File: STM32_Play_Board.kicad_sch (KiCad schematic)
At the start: 0 parts

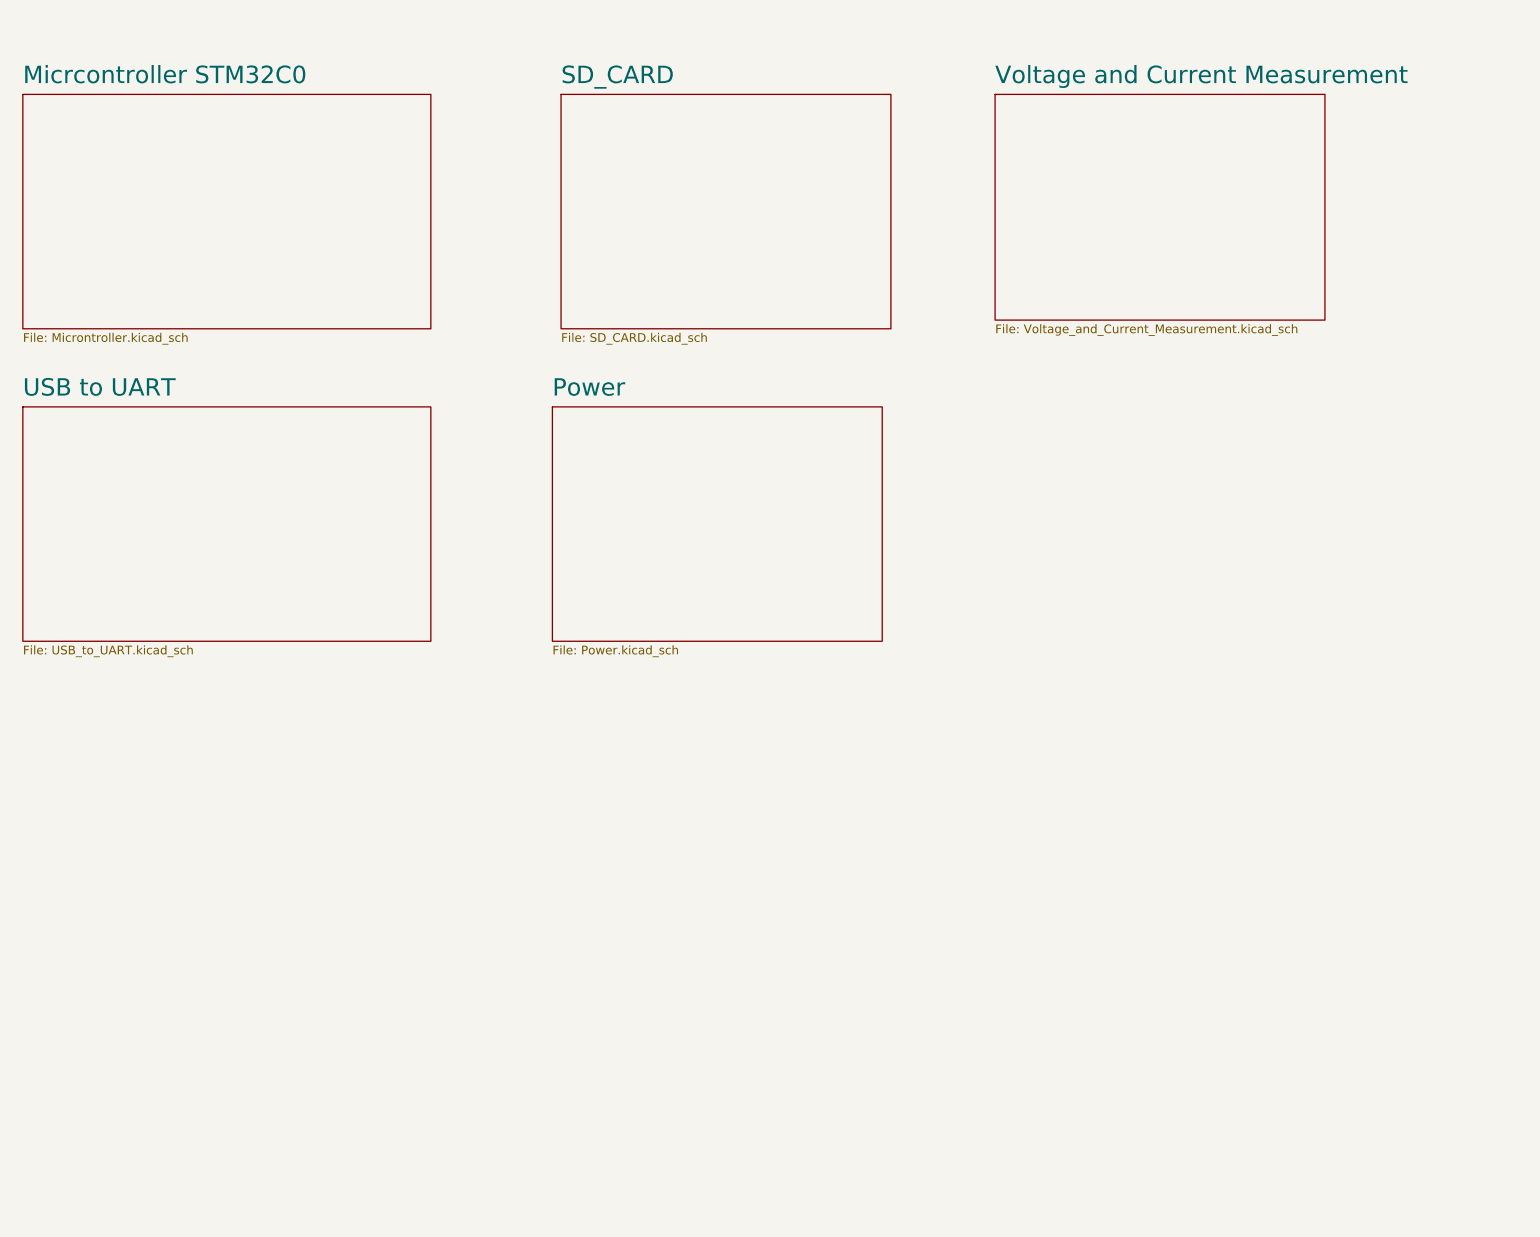
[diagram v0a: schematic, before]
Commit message: changes to schematic and PCB
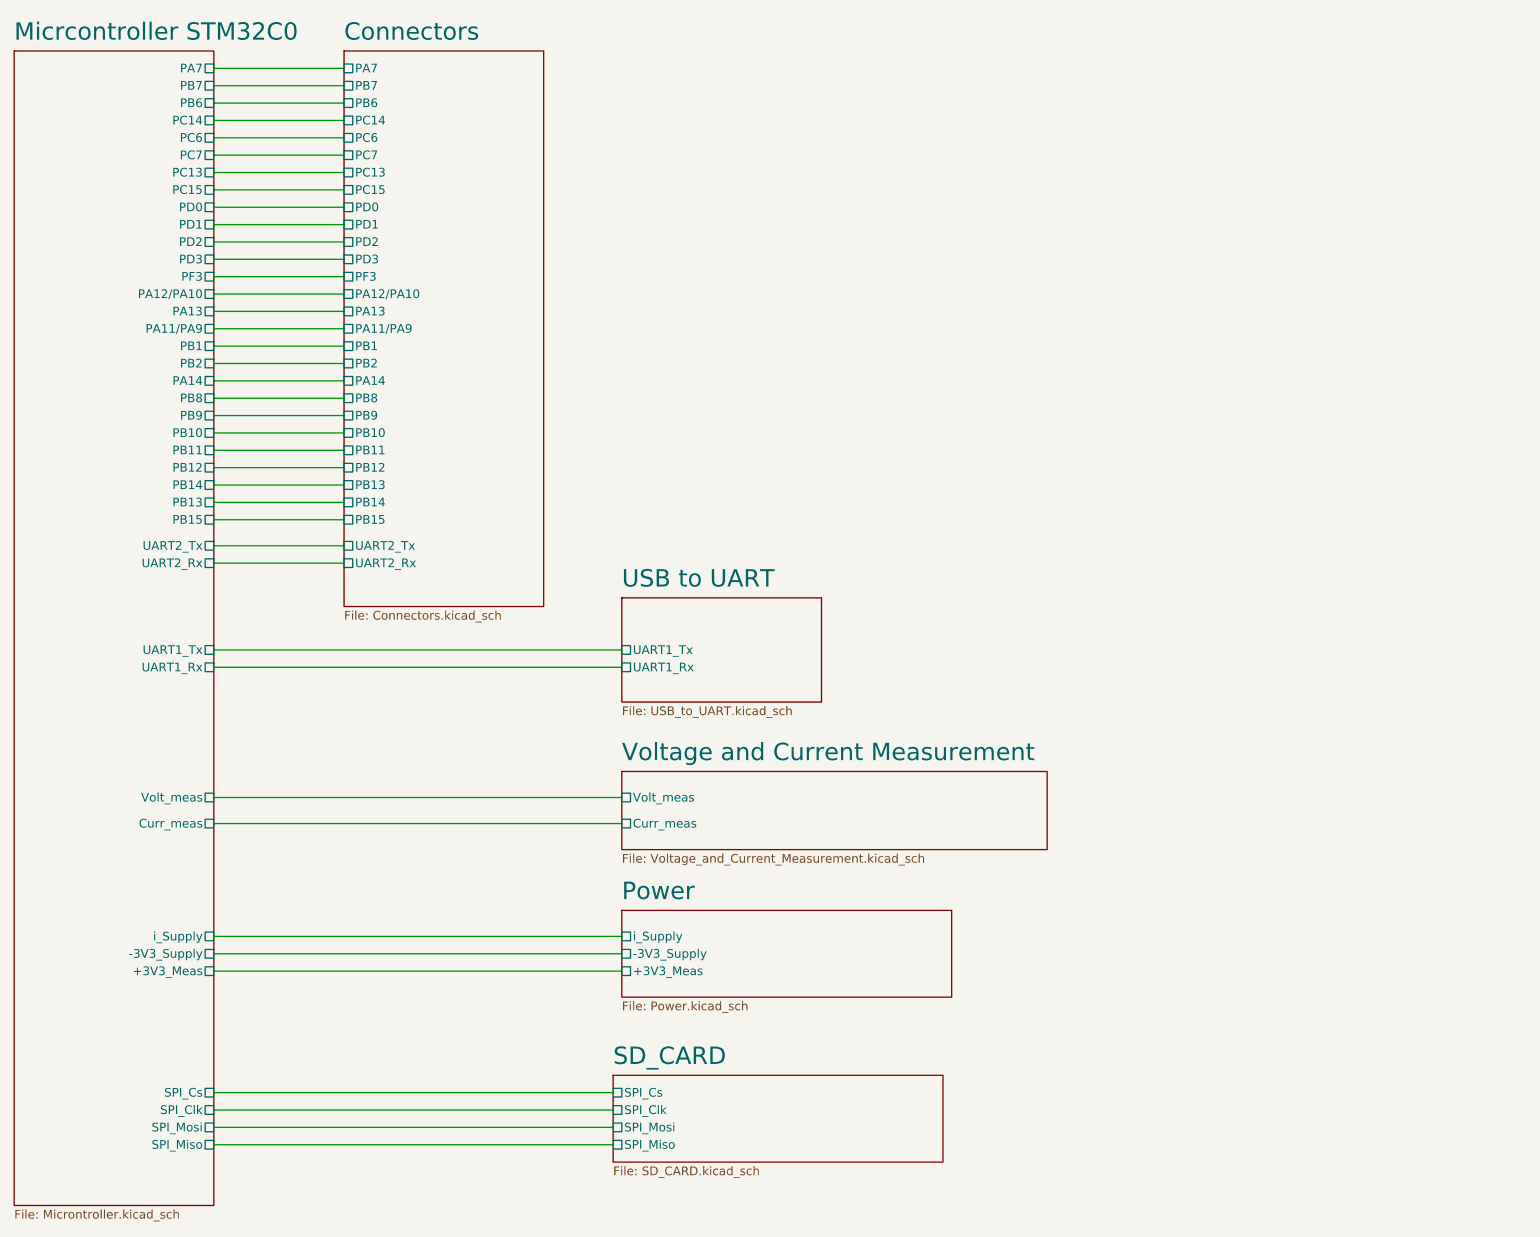
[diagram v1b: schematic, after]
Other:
- added sheet Connectors (Connectors.kicad_sch)
- sheet Micrcontroller STM32C0 ports: added +3V3_Meas, -3V3_Supply, Curr_meas, PA11/PA9, PA12/PA10, PA13, PA14, PA7, PB1, PB10, PB11, PB12, PB13, PB14, PB15, PB2, PB6, PB7, PB8, PB9, PC13, PC14, PC15, PC6, PC7, PD0, PD1, PD2, PD3, PF3, SPI_Clk, SPI_Cs, SPI_Miso, SPI_Mosi, UART1_Rx, UART1_Tx, UART2_Rx, UART2_Tx, Volt_meas, i_Supply; removed none
- sheet Power ports: added +3V3_Meas, -3V3_Supply, i_Supply; removed none
- sheet SD_CARD ports: added SPI_Clk, SPI_Cs, SPI_Miso, SPI_Mosi; removed none
- sheet USB to UART ports: added UART1_Rx, UART1_Tx; removed none
- sheet Voltage and Current Measurement ports: added Curr_meas, Volt_meas; removed none
